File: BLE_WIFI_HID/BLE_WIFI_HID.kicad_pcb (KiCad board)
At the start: 2 copper layers, 62.9 x 33.4 mm, 25 parts, among them J1 Conn_02x03_Odd_Even, J2 Conn_02x03_Odd_Even, P3 PROGRAMMER SERIAL, P4 Battery, U1 ESP32-WROOM, U2 AP2112K-3.3TRG1, U3 MCP73831T-2ACI/OT

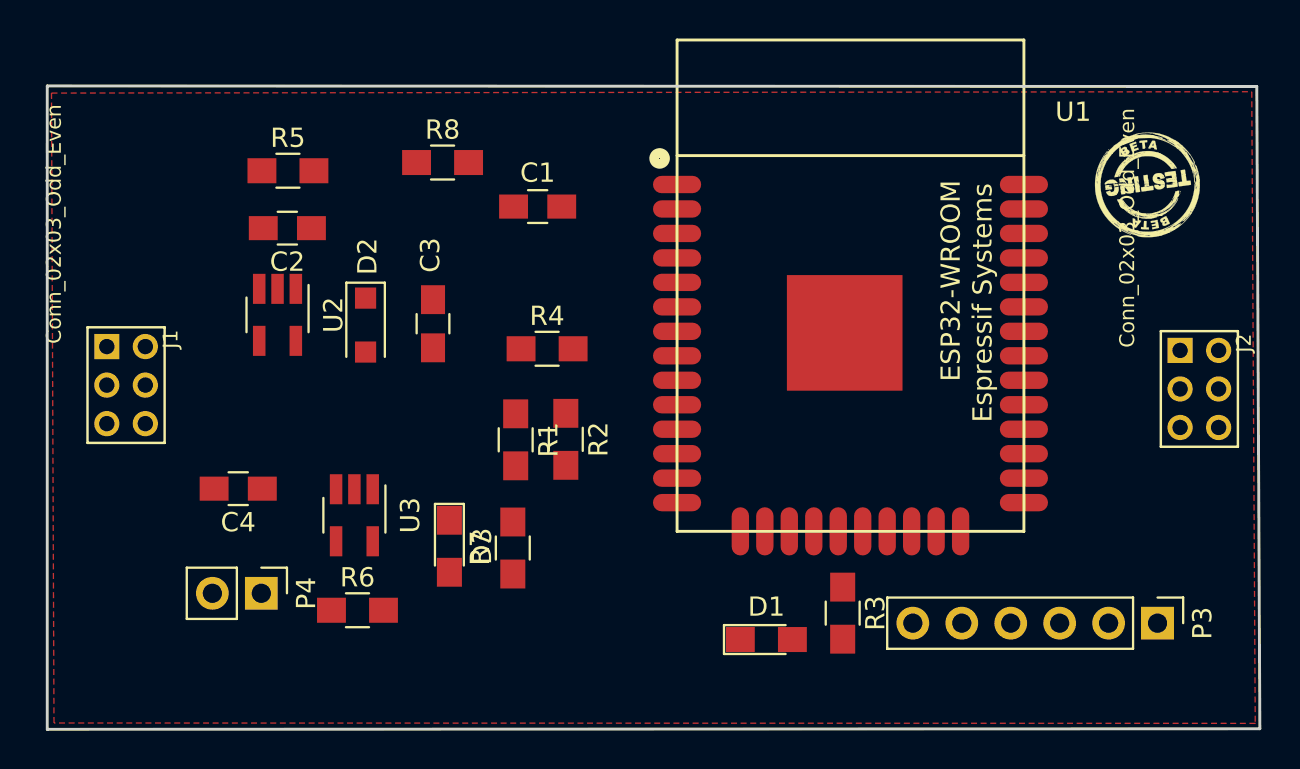
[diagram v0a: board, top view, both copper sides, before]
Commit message: Inicio routeo
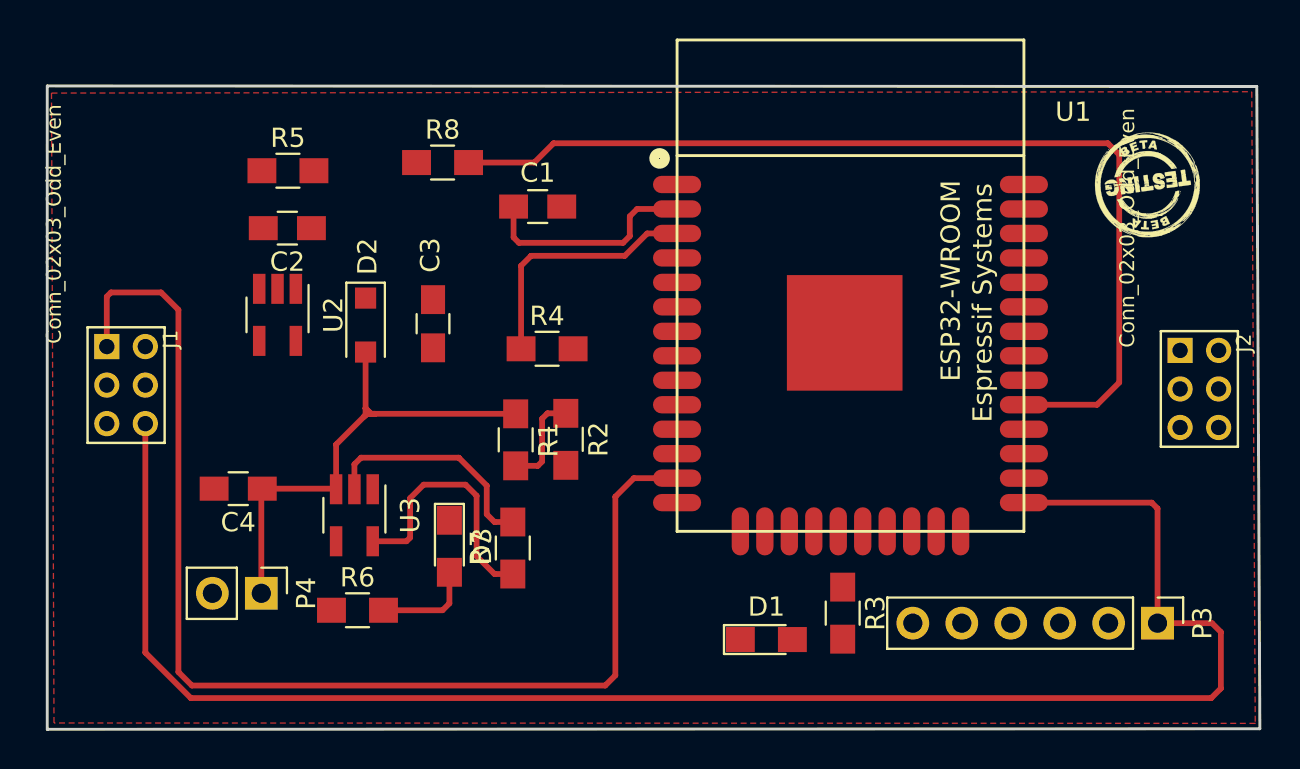
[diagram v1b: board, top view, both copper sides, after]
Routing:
- net /ESP_GPIO0: track 0.00 -> 89.1 mm
- net /MOSI: track 0.00 -> 61.6 mm
- net /ESP_CS: track 0.00 -> 51.7 mm
- net +BATT: track 0.00 -> 25.8 mm
- net Net-(R7-Pad1): track 0.00 -> 13.4 mm
- net /ESP_RESET: track 0.00 -> 13.1 mm
- net Net-(R7-Pad2): track 0.00 -> 11.9 mm
- net +3V3: track 0.00 -> 11.5 mm
- net Net-(D3-Pad2): track 0.00 -> 5.18 mm
- net /AN35_BAT: track 0.00 -> 5.03 mm
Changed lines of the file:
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@@
-(kicad_pcb (version 20171130) (host pcbnew "(5.0.1-3-g963ef8bb5)")
+(kicad_pcb (version 20171130) (host pcbnew "(5.1.2)-2")
   (general
     (thickness 1.6)
     (drawings 5)
-    (tracks 1)
+    (tracks 83)
     (zones 0)
     (modules 25)
@@
     (zone_45_only no)
     (trace_min 0.2)
-    (segment_width 0.2)
-    (edge_width 0.15)
     (via_size 0.6)
     (via_drill 0.4)
@@
     (uvia_min_size 0.2)
     (uvia_min_drill 0.1)
+    (edge_width 0.15)
+    (segment_width 0.2)
     (pcb_text_width 0.3)
     (pcb_text_size 1.5 1.5)
@@
   (gr_line (start 208.648 110.668) (end 145.718 110.698) (layer Edge.Cuts) (width 0.15))
   (gr_line (start 208.488 77.338) (end 208.648 110.668) (layer Edge.Cuts) (width 0.15))
+  (segment (start 175.6 85.45) (end 170.2 85.45) (width 0.3) (layer F.Cu) (net 1))
+  (segment (start 169.918 85.168) (end 169.918 83.568) (width 0.3) (layer F.Cu) (net 1))
+  (segment (start 170.2 85.45) (end 169.918 85.168) (width 0.3) (layer F.Cu) (net 1))
+  (segment (start 175.95 84.075) (end 175.95 85.1) (width 0.3) (layer F.Cu) (net 1))
+  (segment (start 176.332 83.693) (end 175.95 84.075) (width 0.3) (layer F.Cu) (net 1))
+  (segment (start 178.403 83.693) (end 176.332 83.693) (width 0.3) (layer F.Cu) (net 1))
+  (segment (start 175.95 85.1) (end 175.6 85.45) (width 0.3) (layer F.Cu) (net 1))
+  (segment (start 160.678 98.208) (end 160.708 98.238) (width 0.3) (layer F.Cu) (net 4))
+  (segment (start 156.878 98.208) (end 160.678 98.208) (width 0.3) (layer F.Cu) (net 4))
+  (segment (start 156.828 98.258) (end 156.878 98.208) (width 0.3) (layer F.Cu) (net 4))
+  (segment (start 156.828 103.638) (end 156.828 98.258) (width 0.3) (layer F.Cu) (net 4))
+  (segment (start 162.238 94.038) (end 162.238 91.118) (width 0.3) (layer F.Cu) (net 4))
+  (segment (start 160.708 98.238) (end 160.708 95.917) (width 0.3) (layer F.Cu) (net 4))
+  (segment (start 162.523 94.323) (end 162.4125 94.2125) (width 0.3) (layer F.Cu) (net 4))
+  (segment (start 162.4125 94.2125) (end 162.238 94.038) (width 0.3) (layer F.Cu) (net 4))
+  (segment (start 162.2375 94.0385) (end 162.238 94.038) (width 0.3) (layer F.Cu) (net 4))
+  (segment (start 162.2375 94.3875) (end 162.2375 94.0385) (width 0.3) (layer F.Cu) (net 4))
+  (segment (start 162.2375 94.3875) (end 162.4125 94.2125) (width 0.3) (layer F.Cu) (net 4))
+  (segment (start 162.302 94.323) (end 162.15 94.475) (width 0.3) (layer F.Cu) (net 4))
+  (segment (start 162.727 94.323) (end 162.302 94.323) (width 0.3) (layer F.Cu) (net 4))
+  (segment (start 162.15 94.475) (end 162.2375 94.3875) (width 0.3) (layer F.Cu) (net 4))
+  (segment (start 160.708 95.917) (end 162.15 94.475) (width 0.3) (layer F.Cu) (net 4))
+  (segment (start 170.028 94.323) (end 162.727 94.323) (width 0.3) (layer F.Cu) (net 4))
+  (segment (start 162.727 94.323) (end 162.523 94.323) (width 0.3) (layer F.Cu) (net 4))
   (segment (start 184.408 106.018) (end 184.388 106.038) (width 0.3) (layer F.Cu) (net 5))
+  (segment (start 163.168 104.518) (end 166.232 104.518) (width 0.3) (layer F.Cu) (net 7))
+  (segment (start 166.588 104.162) (end 166.588 102.548) (width 0.3) (layer F.Cu) (net 7))
+  (segment (start 166.232 104.518) (end 166.588 104.162) (width 0.3) (layer F.Cu) (net 7))
+  (segment (start 178.403 97.663) (end 176.162 97.663) (width 0.3) (layer F.Cu) (net 8))
+  (segment (start 176.162 97.663) (end 175.2 98.625) (width 0.3) (layer F.Cu) (net 8))
+  (segment (start 175.2 98.625) (end 175.2 107.9) (width 0.3) (layer F.Cu) (net 8))
+  (segment (start 175.2 107.9) (end 174.675 108.425) (width 0.3) (layer F.Cu) (net 8))
+  (segment (start 174.675 108.425) (end 153.225 108.425) (width 0.3) (layer F.Cu) (net 8))
+  (segment (start 153.225 108.425) (end 152.525 107.725) (width 0.3) (layer F.Cu) (net 8))
+  (segment (start 152.525 107.725) (end 152.525 88.925) (width 0.3) (layer F.Cu) (net 8))
+  (segment (start 152.525 88.925) (end 151.625 88.025) (width 0.3) (layer F.Cu) (net 8))
+  (segment (start 151.625 88.025) (end 149.025 88.025) (width 0.3) (layer F.Cu) (net 8))
+  (segment (start 148.808 88.242) (end 148.808 90.833) (width 0.3) (layer F.Cu) (net 8))
+  (segment (start 149.025 88.025) (end 148.808 88.242) (width 0.3) (layer F.Cu) (net 8))
+  (segment (start 171.678 94.298) (end 171.4 94.576) (width 0.3) (layer F.Cu) (net 11))
+  (segment (start 172.628 94.298) (end 171.678 94.298) (width 0.3) (layer F.Cu) (net 11))
+  (segment (start 171.4 94.576) (end 171.4 96.8) (width 0.3) (layer F.Cu) (net 11))
+  (segment (start 171.177 97.023) (end 170.028 97.023) (width 0.3) (layer F.Cu) (net 11))
+  (segment (start 171.4 96.8) (end 171.177 97.023) (width 0.3) (layer F.Cu) (net 11))
+  (segment (start 168.928 102.638) (end 168 101.71) (width 0.3) (layer F.Cu) (net 13))
+  (segment (start 169.878 102.638) (end 168.928 102.638) (width 0.3) (layer F.Cu) (net 13))
+  (segment (start 168 101.71) (end 168 98.575) (width 0.3) (layer F.Cu) (net 13))
+  (segment (start 168 98.575) (end 167.425 98) (width 0.3) (layer F.Cu) (net 13))
+  (segment (start 167.425 98) (end 165.25 98) (width 0.3) (layer F.Cu) (net 13))
+  (segment (start 165.25 98) (end 164.55 98.7) (width 0.3) (layer F.Cu) (net 13))
+  (segment (start 164.55 98.7) (end 164.55 100.75) (width 0.3) (layer F.Cu) (net 13))
+  (segment (start 164.362 100.938) (end 162.608 100.938) (width 0.3) (layer F.Cu) (net 13))
+  (segment (start 164.55 100.75) (end 164.362 100.938) (width 0.3) (layer F.Cu) (net 13))
+  (segment (start 168.928 99.938) (end 168.525 99.535) (width 0.3) (layer F.Cu) (net 14))
+  (segment (start 169.878 99.938) (end 168.928 99.938) (width 0.3) (layer F.Cu) (net 14))
+  (segment (start 168.525 99.535) (end 168.525 98.05) (width 0.3) (layer F.Cu) (net 14))
+  (segment (start 168.525 98.05) (end 167.075 96.6) (width 0.3) (layer F.Cu) (net 14))
+  (segment (start 167.075 96.6) (end 162 96.6) (width 0.3) (layer F.Cu) (net 14))
+  (segment (start 161.658 96.942) (end 161.658 98.238) (width 0.3) (layer F.Cu) (net 14))
+  (segment (start 162 96.6) (end 161.658 96.942) (width 0.3) (layer F.Cu) (net 14))
+  (segment (start 196.403 98.933) (end 203.033 98.933) (width 0.3) (layer F.Cu) (net 36))
+  (segment (start 203.338 99.238) (end 203.338 105.188) (width 0.3) (layer F.Cu) (net 36))
+  (segment (start 203.033 98.933) (end 203.338 99.238) (width 0.3) (layer F.Cu) (net 36))
+  (segment (start 196.403 98.933) (end 197.203 98.933) (width 0.3) (layer F.Cu) (net 36))
+  (segment (start 150.808 106.715122) (end 150.808 94.833) (width 0.3) (layer F.Cu) (net 36))
+  (segment (start 206.163 105.188) (end 206.625 105.65) (width 0.3) (layer F.Cu) (net 36))
+  (segment (start 203.338 105.188) (end 206.163 105.188) (width 0.3) (layer F.Cu) (net 36))
+  (segment (start 206.625 105.65) (end 206.625 108.575) (width 0.3) (layer F.Cu) (net 36))
+  (segment (start 206.625 108.575) (end 206.125 109.075) (width 0.3) (layer F.Cu) (net 36))
+  (segment (start 206.125 109.075) (end 153.167878 109.075) (width 0.3) (layer F.Cu) (net 36))
+  (segment (start 153.167878 109.075) (end 150.808 106.715122) (width 0.3) (layer F.Cu) (net 36))
+  (segment (start 176.853 84.963) (end 175.691 86.125) (width 0.3) (layer F.Cu) (net 37))
+  (segment (start 178.403 84.963) (end 176.853 84.963) (width 0.3) (layer F.Cu) (net 37))
+  (segment (start 175.691 86.125) (end 170.825 86.125) (width 0.3) (layer F.Cu) (net 37))
+  (segment (start 170.308 86.642) (end 170.308 90.948) (width 0.3) (layer F.Cu) (net 37))
+  (segment (start 170.825 86.125) (end 170.308 86.642) (width 0.3) (layer F.Cu) (net 37))
+  (segment (start 196.403 93.853) (end 200.197 93.853) (width 0.3) (layer F.Cu) (net 42))
+  (segment (start 200.197 93.853) (end 201.35 92.7) (width 0.3) (layer F.Cu) (net 42))
+  (segment (start 201.35 92.7) (end 201.35 80.875) (width 0.3) (layer F.Cu) (net 42))
+  (segment (start 200.757999 80.282999) (end 171.992001 80.282999) (width 0.3) (layer F.Cu) (net 42))
+  (segment (start 201.35 80.875) (end 200.757999 80.282999) (width 0.3) (layer F.Cu) (net 42))
+  (segment (start 170.992 81.283) (end 167.583 81.283) (width 0.3) (layer F.Cu) (net 42))
+  (segment (start 171.992001 80.282999) (end 170.992 81.283) (width 0.3) (layer F.Cu) (net 42))
   (zone (net 2) (net_name GND) (layer F.Cu) (hatch edge 0.508)
     (connect_pads (clearance 0.508))
     (min_thickness 0.254)
-    (fill yes (arc_segments 16) (thermal_gap 0.508) (thermal_bridge_width 0.508))
+    (fill (arc_segments 16) (thermal_gap 0.508) (thermal_bridge_width 0.508))
     (polygon
       (pts
